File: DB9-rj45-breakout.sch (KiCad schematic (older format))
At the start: 2 parts, among them CN1 1x9, CN2 1x8

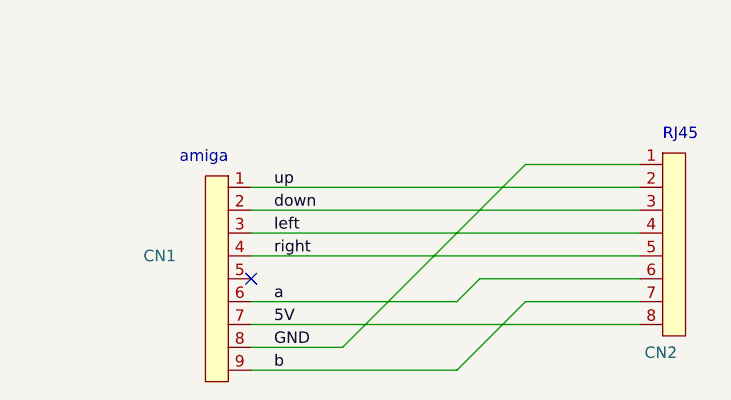
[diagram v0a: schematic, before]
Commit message: b toggle conf
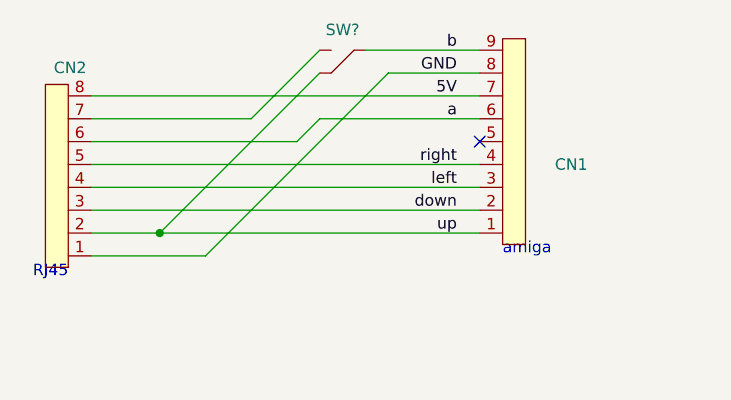
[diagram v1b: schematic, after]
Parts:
- added SW?: spdt, symbol switches:spdt
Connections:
- net b: now also SW?.2 (c); no longer CN2.7
- net up: now also SW?.3 (nc)
- new net: CN2.7, SW?.1 (no)
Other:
- moved on the sheet: CN1, CN2
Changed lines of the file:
@@
 L pin_headers:1x9 CN1
 U 1 1 5FBFEB21
-P 5000 3700
-F 0 "CN1" H 5400 3700 50  0000 C CNN
-F 1 "1x9" H 5000 4100 50  0001 C CNN
-F 2 "connectors:DB9" H 5000 4000 50  0001 C CNN
-F 3 "" H 5000 3800 50  0001 C CNN
-	1    5000 3700
-	-1   0    0    -1
+P 6000 3300
+F 0 "CN1" H 6400 3300 50  0000 C CNN
+F 1 "1x9" H 6000 3700 50  0001 C CNN
+F 2 "connectors:DB9" H 6000 3600 50  0001 C CNN
+F 3 "" H 6000 3400 50  0001 C CNN
+	1    6000 3300
+	1    0    0    1
 $EndComp
 Wire Wire Line
-	5000 4100 5400 4100
+	6000 2900 5600 2900
 Wire Wire Line
-	6200 3300 6700 3300
-Text Label 5100 4100 0    50   ~ 0
+	4800 3700 4300 3700
+Text Label 5900 2900 2    50   ~ 0
 GND
-Text Label 5100 4000 0    50   ~ 0
+Text Label 5900 3000 2    50   ~ 0
 5V
-Text Label 5100 3400 0    50   ~ 0
+Text Label 5900 3600 2    50   ~ 0
 up
-Text Label 5100 3500 0    50   ~ 0
+Text Label 5900 3500 2    50   ~ 0
 down
-Text Label 5100 3600 0    50   ~ 0
+Text Label 5900 3400 2    50   ~ 0
 left
-Text Label 5100 3700 0    50   ~ 0
+Text Label 5900 3300 2    50   ~ 0
 right
-Text Label 5100 3900 0    50   ~ 0
+Text Label 5900 3100 2    50   ~ 0
 a
-Text Label 5100 4200 0    50   ~ 0
+Text Label 5900 2800 2    50   ~ 0
 b
-NoConn ~ 5000 3800
+NoConn ~ 6000 3200
 Wire Wire Line
-	5000 3400 6700 3400
+	6000 3500 4300 3500
 Wire Wire Line
-	5000 3500 6700 3500
+	4300 3400 6000 3400
 Wire Wire Line
-	6700 3600 5000 3600
+	6000 3300 4300 3300
 Wire Wire Line
-	5000 3700 6700 3700
+	5600 2900 4800 3700
 Wire Wire Line
-	5400 4100 6200 3300
-Wire Wire Line
-	5000 4000 6700 4000
-Wire Wire Line
-	6000 3800 6700 3800
-Wire Wire Line
-	5900 4200 6200 3900
-Wire Wire Line
-	6200 3900 6700 3900
-Wire Wire Line
-	5000 4200 5900 4200
-Wire Wire Line
-	5900 3900 6000 3800
-Wire Wire Line
-	5000 3900 5900 3900
-Text Notes 4900 3300 2    50   ~ 0
+	6000 3000 4300 3000
+Text Notes 6100 3700 0    50   ~ 0
 amiga
-Text Notes 6800 3200 0    50   ~ 0
+Text Notes 4200 3800 2    50   ~ 0
 RJ45
 $Comp
 L pin_headers:1x8 CN2
 U 1 1 5FBFEFE7
-P 6700 3600
-F 0 "CN2" H 6792 3077 50  0000 C CNN
-F 1 "1x8" H 6700 4000 50  0001 C CNN
-F 2 "modular-jack:RJHSE-5080" H 6700 3900 50  0001 C CNN
-F 3 "" H 6700 3700 50  0001 C CNN
-	1    6700 3600
-	1    0    0    -1
+P 4300 3400
+F 0 "CN2" H 4392 2877 50  0000 C CNN
+F 1 "1x8" H 4300 3800 50  0001 C CNN
+F 2 "modular-jack:RJHSE-5080" H 4300 3700 50  0001 C CNN
+F 3 "" H 4300 3500 50  0001 C CNN
+	1    4300 3400
+	-1   0    0    1
 $EndComp
+Wire Wire Line
+	5200 3200 4300 3200
+Wire Wire Line
+	6000 3100 5300 3100
+Wire Wire Line
+	5300 3100 5200 3200
+$Comp
+L switches:spdt SW?
+U 1 1 5FD40BAE
+P 5400 2800
+F 0 "SW?" H 5400 2711 50  0000 C CNN
+F 1 "spdt" H 5400 2900 50  0001 C CNN
+F 2 "" H 5400 2800 50  0001 C CNN
+F 3 "" H 5400 2800 50  0001 C CNN
+	1    5400 2800
+	-1   0    0    1
+$EndComp
+Wire Wire Line
+	6000 2800 5500 2800
+Wire Wire Line
+	6000 3600 4600 3600
+Wire Wire Line
+	5300 2900 4600 3600
+Connection ~ 4600 3600
+Wire Wire Line
+	4600 3600 4300 3600
+Wire Wire Line
+	5300 2800 5000 3100
+Wire Wire Line
+	4300 3100 5000 3100
 $EndSCHEMATC
